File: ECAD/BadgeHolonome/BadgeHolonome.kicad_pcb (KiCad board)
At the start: 2 copper layers, 34.8 x 39.9 mm, 3 parts

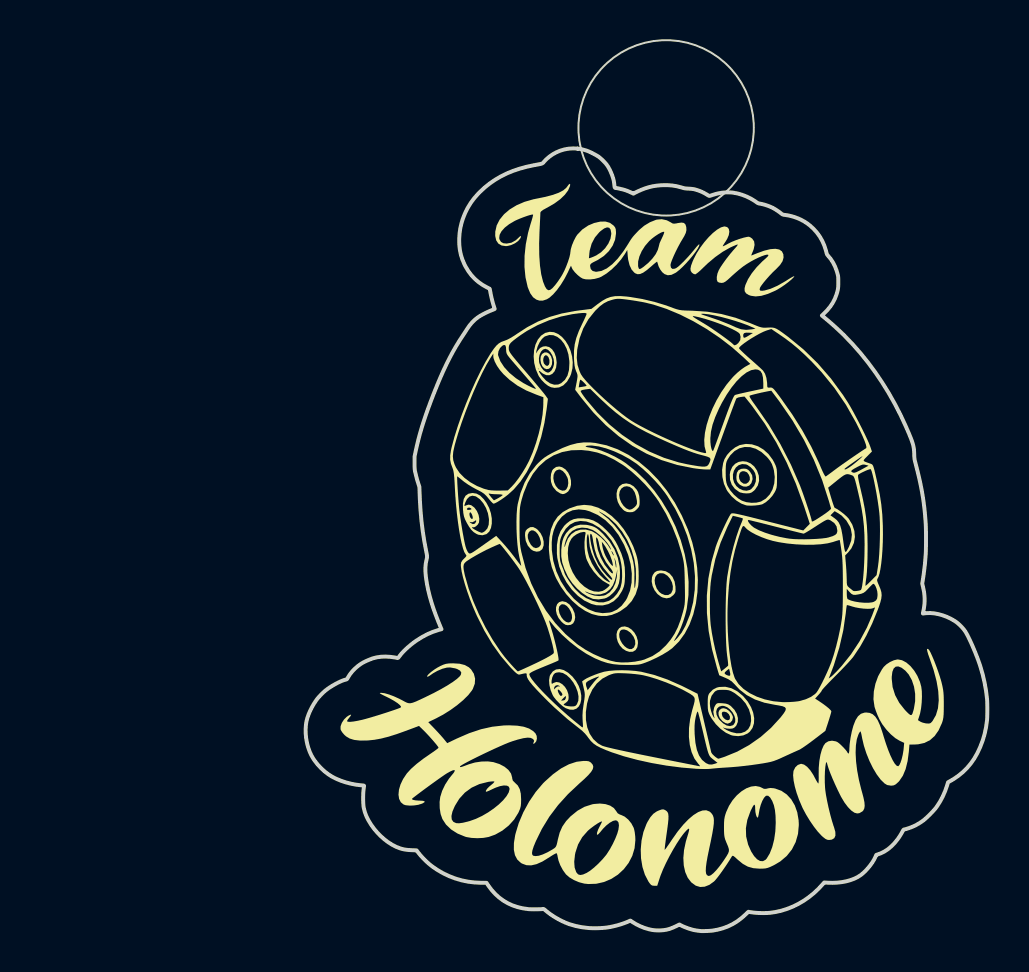
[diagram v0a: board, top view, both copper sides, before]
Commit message: New features
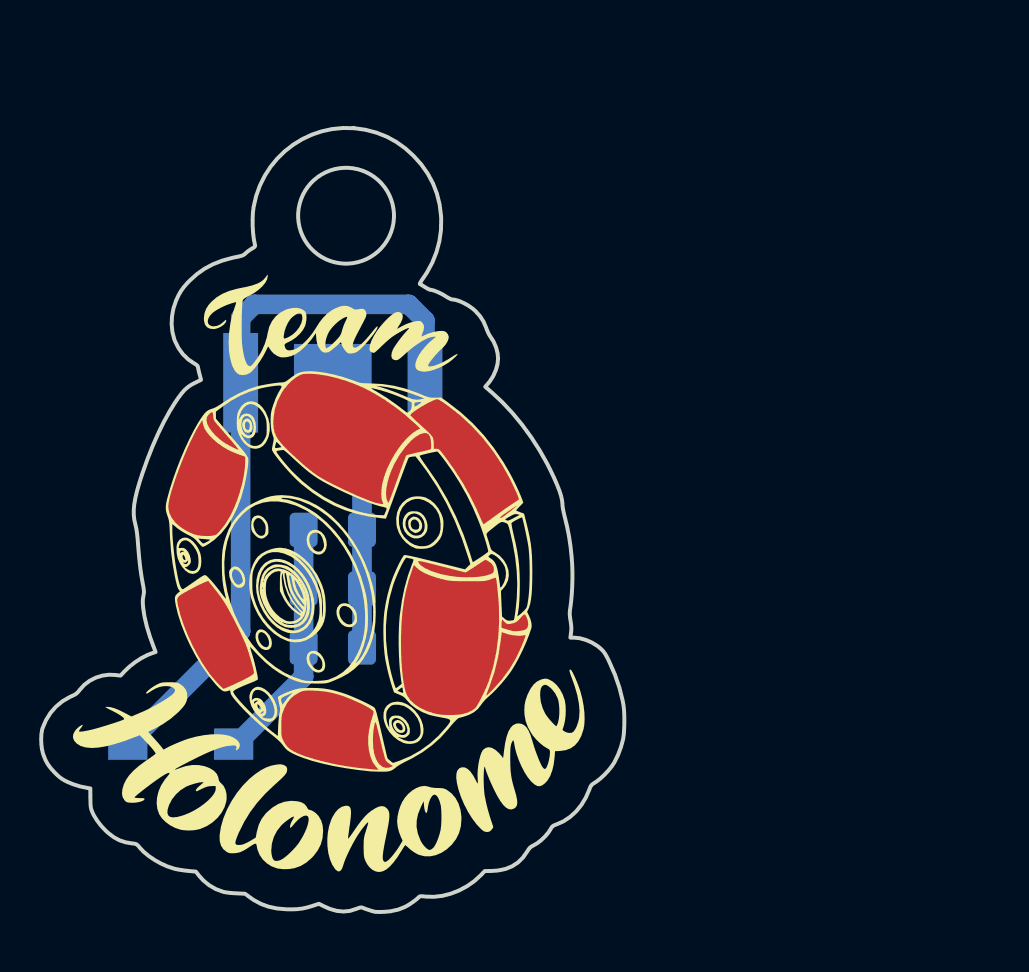
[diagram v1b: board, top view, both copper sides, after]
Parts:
- removed G*** (x3): LOGO, LOGO
- added BT1: Battery_Cell, Battery:BatteryHolder_Keystone_2998_1x6.8mm, B.Cu at (125.0, 73.0)
- added D1: LED_Small, LED_SMD:LED_1206_3216Metric_Pad1.42x1.75mm_HandSolder, B.Cu at (125.0, 86.5)
- added D2: LED_Small, LED_SMD:LED_1206_3216Metric_Pad1.42x1.75mm_HandSolder, B.Cu at (125.0, 80.5)
- added D3: LED_Small, LED_SMD:LED_1206_3216Metric_Pad1.42x1.75mm_HandSolder, B.Cu at (125.0, 83.5)
- added REF**: BadgeHolonome, Badges:BadgeHolonome, F.Cu at (125.0, 80.0)
- added SW1: SW_Push, Button_Switch_SMD:SW_SPST_EVQPE1, B.Cu at (117.2, 91.4)
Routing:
- net Net-(BT1-+): track 0.00 -> 37.3 mm
- net Net-(BT1--): track 0.00 -> 14.1 mm
- net Net-(D1-A): track 0.00 -> 12.5 mm
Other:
- board size 34.8 x 39.9 mm -> 29.7 x 40 mm
